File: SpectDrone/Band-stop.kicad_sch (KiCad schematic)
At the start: 4 parts

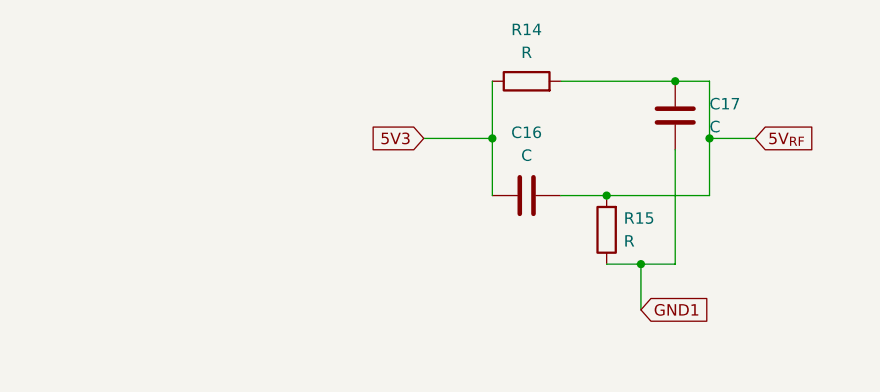
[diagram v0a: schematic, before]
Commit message: SpectDrone Development
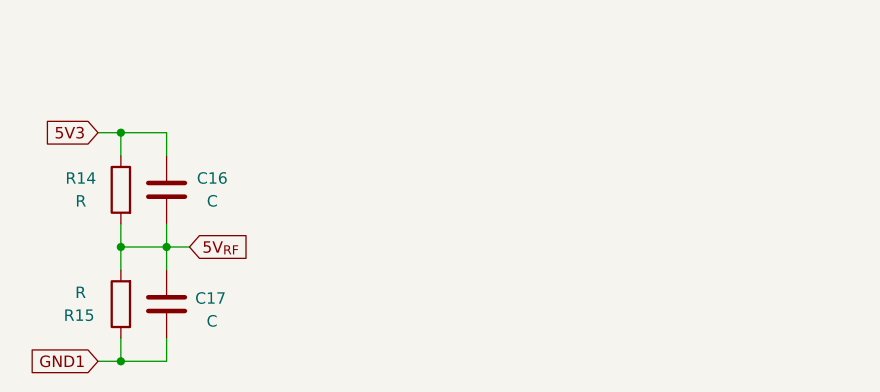
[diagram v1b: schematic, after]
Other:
- moved on the sheet: C16, C17, R14, R15
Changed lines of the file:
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@@
 (kicad_sch (version 20211123) (generator eeschema)
   (paper "A4")
-  (junction (at 142.24 86.36) (diameter 0) (color 0 0 0 0)
+  (junction (at 84.455 97.155) (diameter 0) (color 0 0 0 0)
   )
-  (junction (at 149.86 72.39) (diameter 0) (color 0 0 0 0)
+  (junction (at 89.535 84.455) (diameter 0) (color 0 0 0 0)
   )
-  (junction (at 146.05 66.04) (diameter 0) (color 0 0 0 0)
+  (junction (at 84.455 84.455) (diameter 0) (color 0 0 0 0)
   )
-  (junction (at 138.43 78.74) (diameter 0) (color 0 0 0 0)
+  (junction (at 84.455 71.755) (diameter 0) (color 0 0 0 0)
   )
-  (junction (at 125.73 72.39) (diameter 0) (color 0 0 0 0)
-  )
-  (wire (pts (xy 146.05 86.36) (xy 146.05 73.66))
+  (wire (pts (xy 89.535 94.615) (xy 89.535 97.155))
     (stroke (width 0) (type default) (color 0 0 0 0))
   )
-  (wire (pts (xy 149.86 72.39) (xy 154.94 72.39))
+  (wire (pts (xy 84.455 94.615) (xy 84.455 97.155))
     (stroke (width 0) (type default) (color 0 0 0 0))
   )
-  (wire (pts (xy 138.43 78.74) (xy 149.86 78.74))
+  (wire (pts (xy 89.535 84.455) (xy 92.075 84.455))
     (stroke (width 0) (type default) (color 0 0 0 0))
   )
-  (wire (pts (xy 146.05 66.04) (xy 149.86 66.04))
+  (wire (pts (xy 89.535 84.455) (xy 84.455 84.455))
     (stroke (width 0) (type default) (color 0 0 0 0))
   )
-  (wire (pts (xy 149.86 66.04) (xy 149.86 72.39))
+  (wire (pts (xy 84.455 84.455) (xy 84.455 86.995))
     (stroke (width 0) (type default) (color 0 0 0 0))
   )
-  (wire (pts (xy 142.24 86.36) (xy 142.24 91.44))
+  (wire (pts (xy 84.455 97.155) (xy 81.915 97.155))
     (stroke (width 0) (type default) (color 0 0 0 0))
   )
-  (wire (pts (xy 138.43 86.36) (xy 142.24 86.36))
+  (wire (pts (xy 84.455 97.155) (xy 89.535 97.155))
     (stroke (width 0) (type default) (color 0 0 0 0))
   )
-  (wire (pts (xy 142.24 86.36) (xy 146.05 86.36))
+  (wire (pts (xy 81.915 71.755) (xy 84.455 71.755))
     (stroke (width 0) (type default) (color 0 0 0 0))
   )
-  (wire (pts (xy 125.73 72.39) (xy 125.73 78.74))
+  (wire (pts (xy 89.535 84.455) (xy 89.535 86.995))
     (stroke (width 0) (type default) (color 0 0 0 0))
   )
-  (wire (pts (xy 118.11 72.39) (xy 125.73 72.39))
+  (wire (pts (xy 84.455 81.915) (xy 84.455 84.455))
     (stroke (width 0) (type default) (color 0 0 0 0))
   )
-  (wire (pts (xy 133.35 78.74) (xy 138.43 78.74))
+  (wire (pts (xy 89.535 71.755) (xy 89.535 74.295))
     (stroke (width 0) (type default) (color 0 0 0 0))
   )
-  (wire (pts (xy 125.73 66.04) (xy 125.73 72.39))
+  (wire (pts (xy 84.455 71.755) (xy 89.535 71.755))
     (stroke (width 0) (type default) (color 0 0 0 0))
   )
-  (wire (pts (xy 149.86 72.39) (xy 149.86 78.74))
+  (wire (pts (xy 84.455 71.755) (xy 84.455 74.295))
     (stroke (width 0) (type default) (color 0 0 0 0))
   )
-  (wire (pts (xy 133.35 66.04) (xy 146.05 66.04))
+  (wire (pts (xy 89.535 81.915) (xy 89.535 84.455))
     (stroke (width 0) (type default) (color 0 0 0 0))
   )
-  (global_label "5V_{RF}" (shape input) (at 154.94 72.39 0) (fields_autoplaced)
+  (global_label "5V_{RF}" (shape input) (at 92.075 84.455 0) (fields_autoplaced)
     (effects (font (size 1.27 1.27)) (justify left))
-    (property "Intersheet References" "${INTERSHEET_REFS}" (id 0) (at 161.5381 72.3106 0)
+    (property "Intersheet References" "${INTERSHEET_REFS}" (id 0) (at 98.6731 84.3756 0)
       (effects (font (size 1.27 1.27)) (justify left) hide)
     )
   )
-  (global_label "5V3" (shape input) (at 118.11 72.39 180) (fields_autoplaced)
+  (global_label "5V3" (shape input) (at 81.915 71.755 180) (fields_autoplaced)
     (effects (font (size 1.27 1.27)) (justify right))
-    (property "Intersheet References" "${INTERSHEET_REFS}" (id 0) (at 112.1893 72.4694 0)
+    (property "Intersheet References" "${INTERSHEET_REFS}" (id 0) (at 75.9943 71.8344 0)
       (effects (font (size 1.27 1.27)) (justify right) hide)
     )
   )
-  (global_label "GND1" (shape input) (at 142.24 91.44 0) (fields_autoplaced)
-    (effects (font (size 1.27 1.27)) (justify left))
-    (property "Intersheet References" "${INTERSHEET_REFS}" (id 0) (at 149.7331 91.3606 0)
-      (effects (font (size 1.27 1.27)) (justify left) hide)
+  (global_label "GND1" (shape input) (at 81.915 97.155 180) (fields_autoplaced)
+    (effects (font (size 1.27 1.27)) (justify right))
+    (property "Intersheet References" "${INTERSHEET_REFS}" (id 0) (at 74.4219 97.2344 0)
+      (effects (font (size 1.27 1.27)) (justify right) hide)
     )
   )
-  (symbol (lib_id "Device:C") (at 146.05 69.85 0) (unit 1)
-    (in_bom yes) (on_board yes) (fields_autoplaced)
-    (property "Reference" "C17" (id 0) (at 149.86 68.5799 0)
+  (symbol (lib_id "Device:C") (at 89.535 90.805 0) (unit 1)
+    (in_bom yes) (on_board yes)
+    (property "Reference" "C17" (id 0) (at 92.71 90.17 0)
       (effects (font (size 1.27 1.27)) (justify left))
     )
-    (property "Value" "C" (id 1) (at 149.86 71.1199 0)
+    (property "Value" "C" (id 1) (at 93.98 92.71 0)
       (effects (font (size 1.27 1.27)) (justify left))
     )
-    (property "Footprint" "Capacitor_SMD:C_0603_1608Metric" (id 2) (at 147.0152 73.66 0)
+    (property "Footprint" "Capacitor_SMD:C_0603_1608Metric" (id 2) (at 90.5002 94.615 0)
       (effects (font (size 1.27 1.27)) hide)
     )
-    (property "Datasheet" "~" (id 3) (at 146.05 69.85 0)
+    (property "Datasheet" "~" (id 3) (at 89.535 90.805 0)
       (effects (font (size 1.27 1.27)) hide)
     )
@@
     (pin "2")
   )
-  (symbol (lib_id "Device:R") (at 129.54 66.04 90) (unit 1)
-    (in_bom yes) (on_board yes) (fields_autoplaced)
-    (property "Reference" "R14" (id 0) (at 129.54 60.325 90))
-    (property "Value" "R" (id 1) (at 129.54 62.865 90))
-    (property "Footprint" "Resistor_SMD:R_0603_1608Metric" (id 2) (at 129.54 67.818 90)
+  (symbol (lib_id "Device:R") (at 84.455 78.105 0) (mirror y) (unit 1)
+    (in_bom yes) (on_board yes)
+    (property "Reference" "R14" (id 0) (at 80.01 76.835 0))
+    (property "Value" "R" (id 1) (at 80.01 79.375 0))
+    (property "Footprint" "Resistor_SMD:R_0603_1608Metric" (id 2) (at 86.233 78.105 90)
       (effects (font (size 1.27 1.27)) hide)
     )
-    (property "Datasheet" "~" (id 3) (at 129.54 66.04 0)
+    (property "Datasheet" "~" (id 3) (at 84.455 78.105 0)
       (effects (font (size 1.27 1.27)) hide)
     )
@@
     (pin "2")
   )
-  (symbol (lib_id "Device:C") (at 129.54 78.74 90) (unit 1)
-    (in_bom yes) (on_board yes) (fields_autoplaced)
-    (property "Reference" "C16" (id 0) (at 129.54 71.755 90))
-    (property "Value" "C" (id 1) (at 129.54 74.295 90))
-    (property "Footprint" "Capacitor_SMD:C_0603_1608Metric" (id 2) (at 133.35 77.7748 0)
+  (symbol (lib_id "Device:C") (at 89.535 78.105 0) (mirror y) (unit 1)
+    (in_bom yes) (on_board yes)
+    (property "Reference" "C16" (id 0) (at 94.615 76.835 0))
+    (property "Value" "C" (id 1) (at 94.615 79.375 0))
+    (property "Footprint" "Capacitor_SMD:C_0603_1608Metric" (id 2) (at 88.5698 81.915 0)
       (effects (font (size 1.27 1.27)) hide)
     )
-    (property "Datasheet" "~" (id 3) (at 129.54 78.74 0)
+    (property "Datasheet" "~" (id 3) (at 89.535 78.105 0)
       (effects (font (size 1.27 1.27)) hide)
     )
@@
     (pin "2")
   )
-  (symbol (lib_id "Device:R") (at 138.43 82.55 180) (unit 1)
-    (in_bom yes) (on_board yes) (fields_autoplaced)
-    (property "Reference" "R15" (id 0) (at 140.335 81.2799 0)
+  (symbol (lib_id "Device:R") (at 84.455 90.805 180) (unit 1)
+    (in_bom yes) (on_board yes)
+    (property "Reference" "R15" (id 0) (at 78.105 92.075 0)
       (effects (font (size 1.27 1.27)) (justify right))
     )
-    (property "Value" "R" (id 1) (at 140.335 83.8199 0)
+    (property "Value" "R" (id 1) (at 79.375 89.535 0)
       (effects (font (size 1.27 1.27)) (justify right))
     )
-    (property "Footprint" "Resistor_SMD:R_0603_1608Metric" (id 2) (at 140.208 82.55 90)
+    (property "Footprint" "Resistor_SMD:R_0603_1608Metric" (id 2) (at 86.233 90.805 90)
       (effects (font (size 1.27 1.27)) hide)
     )
-    (property "Datasheet" "~" (id 3) (at 138.43 82.55 0)
+    (property "Datasheet" "~" (id 3) (at 84.455 90.805 0)
       (effects (font (size 1.27 1.27)) hide)
     )
